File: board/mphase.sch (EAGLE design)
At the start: 23 parts, among them IC1 MAX232, IC2 PIC18F4455_40, X1 332-10, X2 332-10

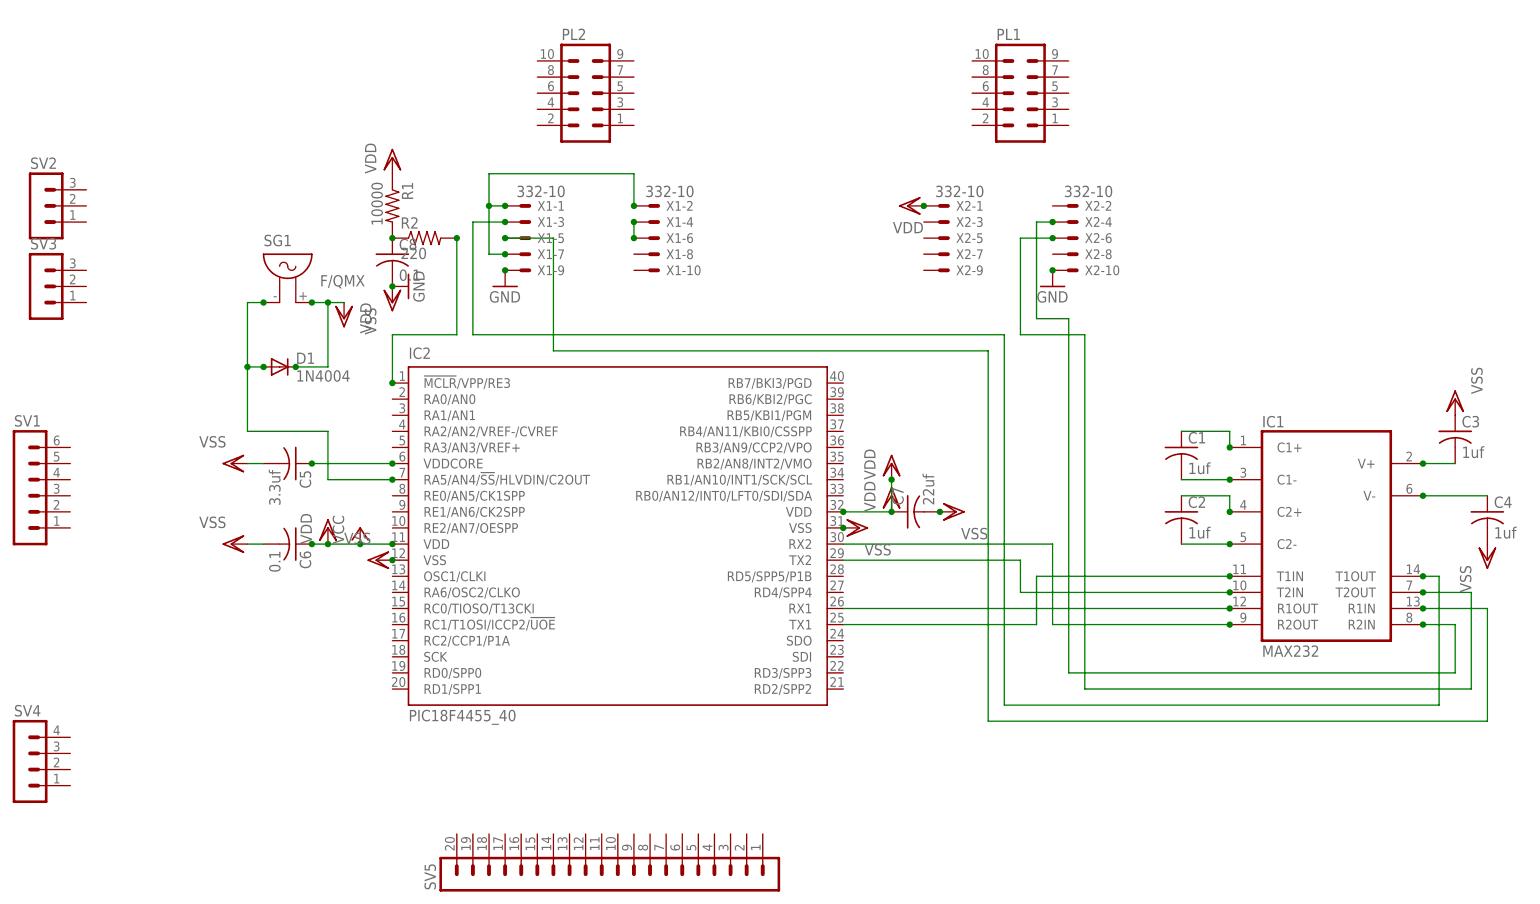
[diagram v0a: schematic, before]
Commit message: update code
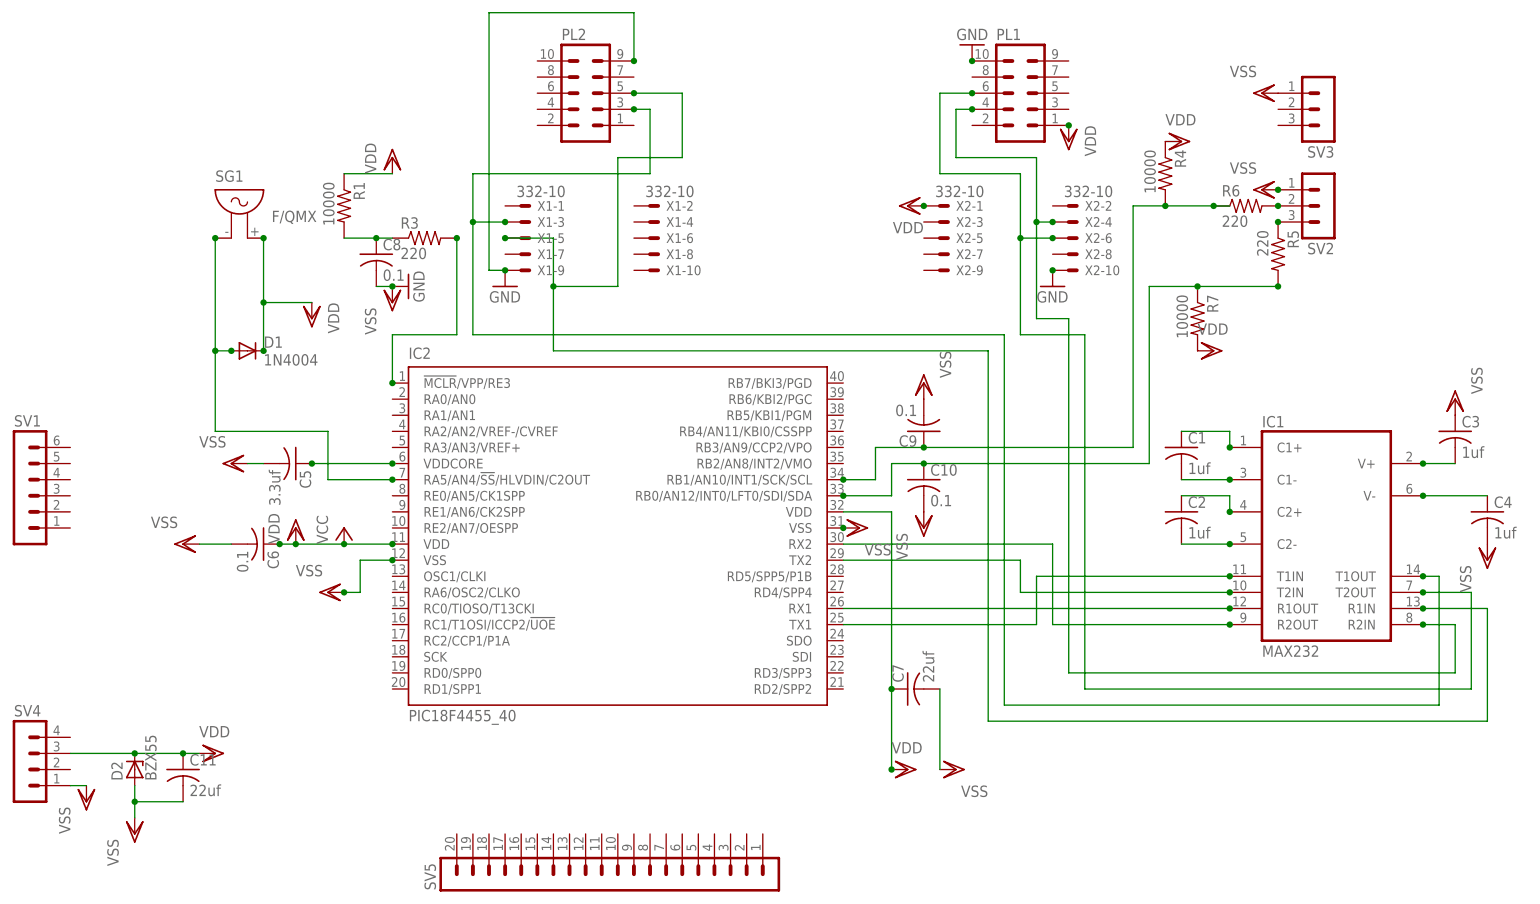
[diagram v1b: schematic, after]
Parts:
- added C10, C9: 0.1, resistor:C-US025-024X044
- added C11: 22uf, resistor:C-US025-025X050
- added D2: BZX55, diode:BZX55
- added R4, R7: 10000, resistor:R-US_0204/2V
- added R5, R6: 220, resistor:R-US_0204/2V
- renumbered R2 to R3
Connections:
- removed net N$15: IC1G$1.R2IN, X2-4.S
- removed net N$18: X1-1.S, X1-2.S, X1-7.S
- new net N$21: C9.1, IC2.RB1/AN10/INT1/SCK/SCL, R4.2, R6.1
- new net N$22: C10.1, IC2.RB0/AN12/INT0/LFT0/SDI/SDA, R5.2, R7.1
- new net N$24: R6.2, SV2.2
- new net N$25: R5.1, SV2.3
- net GND: now also PL1.10, PL2.9
- net N$16: now also PL1.6
- net N$17: now also IC1G$1.R2IN, PL1.4, X2-4.S; no longer X1-4.S, X1-6.S
- net N$19: now also PL2.3
- net N$20: now also PL2.5
- net VDD: now also C11.1, D2.C, PL1.1, R4.1, R7.2, SV4.3
- net VSS: now also C10.2, C11.2, C9.2, D2.A, SV2.1, SV3.1, SV4.1
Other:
- moved on the sheet: C6, C7, C8, D1, R1, SG1, SV2, SV3

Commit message: update code
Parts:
- IC2: MPN (none) -> PIC18F45K80
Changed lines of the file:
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@@
 <grid distance="0.1" unitdist="inch" unit="inch" style="lines" multiple="1" display="no" altdistance="0.01" altunitdist="inch" altunit="inch"/>
 <layers>
-<layer number="1" name="Top" color="4" fill="1" visible="no" active="no"/>
-<layer number="2" name="Route2" color="1" fill="3" visible="no" active="no"/>
-<layer number="3" name="Route3" color="4" fill="3" visible="no" active="no"/>
-<layer number="14" name="Route14" color="1" fill="6" visible="no" active="no"/>
-<layer number="15" name="Route15" color="4" fill="6" visible="no" active="no"/>
-<layer number="16" name="Bottom" color="1" fill="1" visible="no" active="no"/>
-<layer number="17" name="Pads" color="2" fill="1" visible="no" active="no"/>
-<layer number="18" name="Vias" color="2" fill="1" visible="no" active="no"/>
-<layer number="19" name="Unrouted" color="6" fill="1" visible="no" active="no"/>
-<layer number="20" name="Dimension" color="15" fill="1" visible="no" active="no"/>
-<layer number="21" name="tPlace" color="7" fill="1" visible="no" active="no"/>
-<layer number="22" name="bPlace" color="7" fill="1" visible="no" active="no"/>
-<layer number="23" name="tOrigins" color="15" fill="1" visible="no" active="no"/>
-<layer number="24" name="bOrigins" color="15" fill="1" visible="no" active="no"/>
-<layer number="25" name="tNames" color="7" fill="1" visible="no" active="no"/>
-<layer number="26" name="bNames" color="7" fill="1" visible="no" active="no"/>
-<layer number="27" name="tValues" color="7" fill="1" visible="no" active="no"/>
-<layer number="28" name="bValues" color="7" fill="1" visible="no" active="no"/>
+<layer number="1" name="Top" color="4" fill="1" visible="yes" active="no"/>
+<layer number="2" name="Route2" color="1" fill="3" visible="yes" active="no"/>
+<layer number="3" name="Route3" color="4" fill="3" visible="yes" active="no"/>
+<layer number="14" name="Route14" color="1" fill="6" visible="yes" active="no"/>
+<layer number="15" name="Route15" color="4" fill="6" visible="yes" active="no"/>
+<layer number="16" name="Bottom" color="1" fill="1" visible="yes" active="no"/>
+<layer number="17" name="Pads" color="2" fill="1" visible="yes" active="no"/>
+<layer number="18" name="Vias" color="2" fill="1" visible="yes" active="no"/>
+<layer number="19" name="Unrouted" color="6" fill="1" visible="yes" active="no"/>
+<layer number="20" name="Dimension" color="15" fill="1" visible="yes" active="no"/>
+<layer number="21" name="tPlace" color="7" fill="1" visible="yes" active="no"/>
+<layer number="22" name="bPlace" color="7" fill="1" visible="yes" active="no"/>
+<layer number="23" name="tOrigins" color="15" fill="1" visible="yes" active="no"/>
+<layer number="24" name="bOrigins" color="15" fill="1" visible="yes" active="no"/>
+<layer number="25" name="tNames" color="7" fill="1" visible="yes" active="no"/>
+<layer number="26" name="bNames" color="7" fill="1" visible="yes" active="no"/>
+<layer number="27" name="tValues" color="7" fill="1" visible="yes" active="no"/>
+<layer number="28" name="bValues" color="7" fill="1" visible="yes" active="no"/>
 <layer number="29" name="tStop" color="7" fill="3" visible="no" active="no"/>
 <layer number="30" name="bStop" color="7" fill="6" visible="no" active="no"/>
@@
 <layer number="35" name="tGlue" color="7" fill="4" visible="no" active="no"/>
 <layer number="36" name="bGlue" color="7" fill="5" visible="no" active="no"/>
-<layer number="37" name="tTest" color="7" fill="1" visible="no" active="no"/>
-<layer number="38" name="bTest" color="7" fill="1" visible="no" active="no"/>
+<layer number="37" name="tTest" color="7" fill="1" visible="yes" active="no"/>
+<layer number="38" name="bTest" color="7" fill="1" visible="yes" active="no"/>
 <layer number="39" name="tKeepout" color="4" fill="11" visible="no" active="no"/>
 <layer number="40" name="bKeepout" color="1" fill="11" visible="no" active="no"/>
@@
 <layer number="44" name="Drills" color="7" fill="1" visible="no" active="no"/>
 <layer number="45" name="Holes" color="7" fill="1" visible="no" active="no"/>
-<layer number="46" name="Milling" color="3" fill="1" visible="no" active="no"/>
-<layer number="47" name="Measures" color="7" fill="1" visible="no" active="no"/>
-<layer number="48" name="Document" color="7" fill="1" visible="no" active="no"/>
-<layer number="49" name="Reference" color="7" fill="1" visible="no" active="no"/>
-<layer number="51" name="tDocu" color="7" fill="1" visible="no" active="no"/>
-<layer number="52" name="bDocu" color="7" fill="1" visible="no" active="no"/>
+<layer number="46" name="Milling" color="3" fill="1" visible="yes" active="no"/>
+<layer number="47" name="Measures" color="7" fill="1" visible="yes" active="no"/>
+<layer number="48" name="Document" color="7" fill="1" visible="yes" active="no"/>
+<layer number="49" name="Reference" color="7" fill="1" visible="yes" active="no"/>
+<layer number="51" name="tDocu" color="7" fill="1" visible="yes" active="no"/>
+<layer number="52" name="bDocu" color="7" fill="1" visible="yes" active="no"/>
 <layer number="90" name="Modules" color="5" fill="1" visible="yes" active="yes"/>
 <layer number="91" name="Nets" color="2" fill="1" visible="yes" active="yes"/>
@@
 <part name="X1" library="con-garry" deviceset="332-10" device=""/>
 <part name="X2" library="con-garry" deviceset="332-10" device=""/>
-<part name="IC2" library="microchip" deviceset="PIC18F4*_40" device="" technology="455"/>
+<part name="IC2" library="microchip" deviceset="PIC18F4*_40" device="" technology="455">
+<attribute name="MPN" value="PIC18F45K80"/>
+</part>
 <part name="C1" library="resistor" deviceset="C-US" device="025-025X050" value="1uf"/>
 <part name="C2" library="resistor" deviceset="C-US" device="025-025X050" value="1uf"/>
